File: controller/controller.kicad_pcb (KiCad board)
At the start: 2 copper layers, 160 x 100 mm, 8 parts, among them J2 Barrel_Jack_Switch, J3 Conn_01x02, P1 PMOD-Device-x2-Type-Generic-A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, P2 PMOD-Device-x2-Type-Generic-A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, P3 PMOD-Device-x2-Type-Generic-A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, U1 MAX4820xUP, U3 NUCLEO144-F767ZI, U4 TSR_1-2450

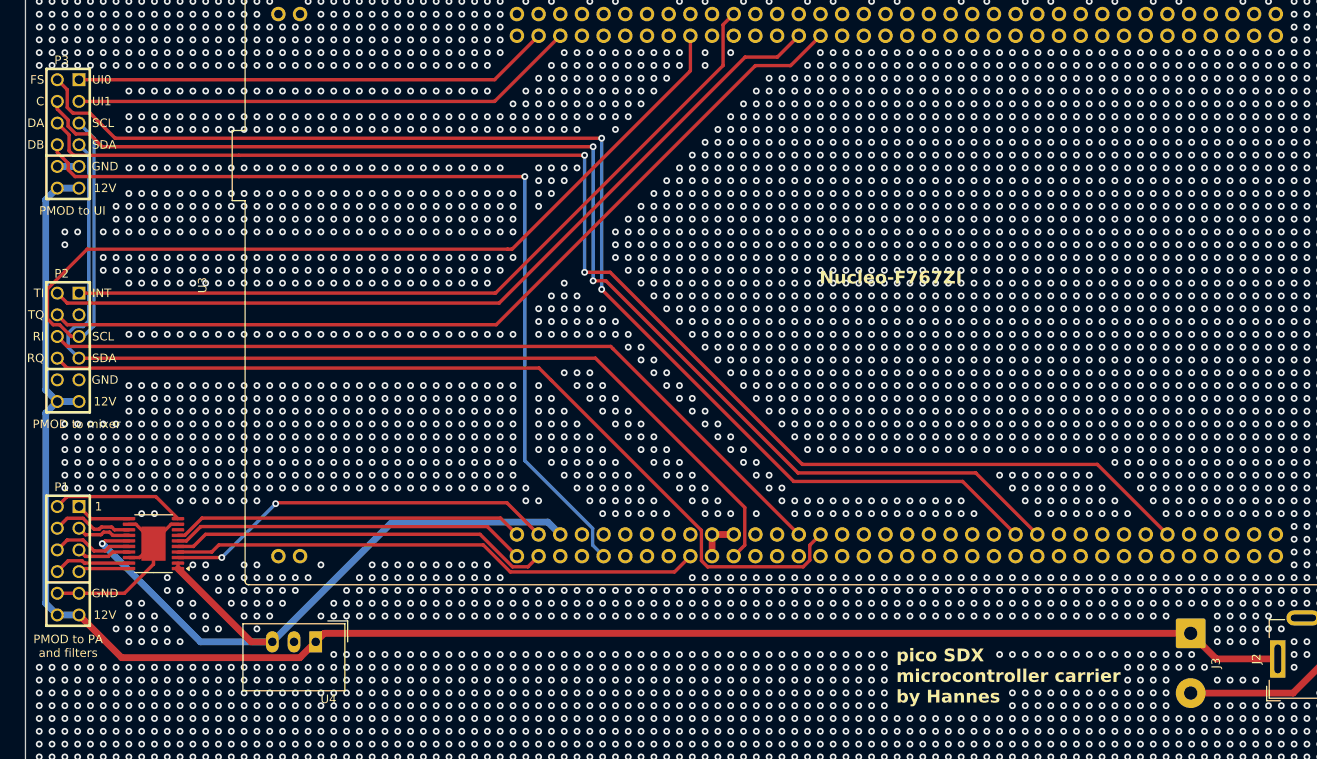
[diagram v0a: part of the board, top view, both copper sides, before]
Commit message: clean up
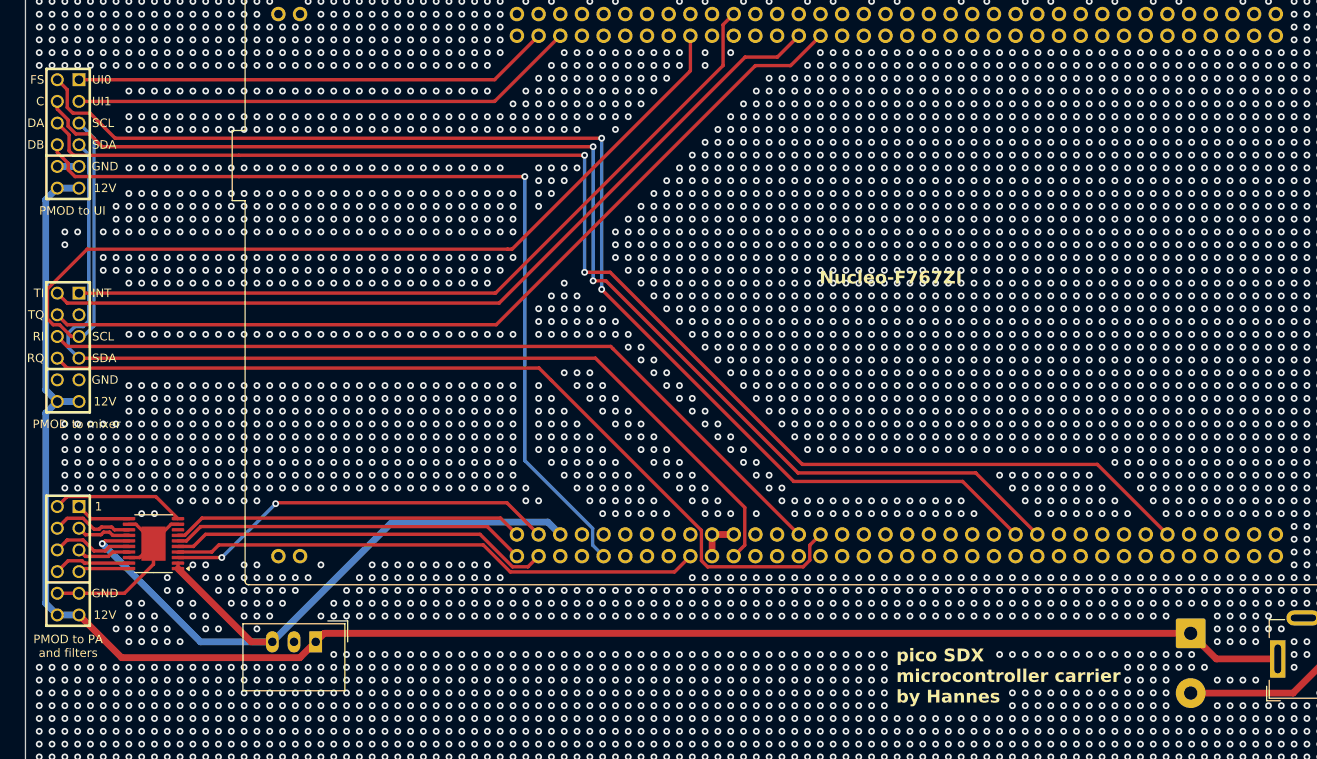
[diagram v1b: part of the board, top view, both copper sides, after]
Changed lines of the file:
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@@
 			(at -1.5 -6.71 0)
 			(layer "F.SilkS")
+			(hide yes)
 			(effects
 				(font
@@
 			(at -0.762 -8.636 0)
 			(layer "F.SilkS")
+			(hide yes)
 			(effects
 				(font
@@
 			(at 3.5 -2.95 90)
 			(layer "F.SilkS")
+			(hide yes)
 			(effects
 				(font
@@
 			(at -0.762 -8.636 0)
 			(layer "F.SilkS")
+			(hide yes)
 			(effects
 				(font
@@
 			(at 0 -2.5 90)
 			(layer "F.SilkS")
+			(hide yes)
 			(effects
 				(font
@@
 			(at -0.762 -8.636 0)
 			(layer "F.SilkS")
+			(hide yes)
 			(effects
 				(font
@@
 			(at 31.75 -36.83 90)
 			(layer "F.SilkS")
+			(hide yes)
 			(effects
 				(font
@@
 		)
 		(height -8)
-		(gr_text "984.2520 mils"
+		(gr_text "25.0000 mm"
 			(at 5.935 42.186 90)
 			(layer "Dwgs.User")
@@
 		)
 		(height -8)
-		(gr_text "984.2520 mils"
+		(gr_text "25.0000 mm"
 			(at 5.935 67.186 90)
 			(layer "Dwgs.User")
@@
 		)
 		(height -8)
-		(gr_text "492.1260 mils"
+		(gr_text "12.5000 mm"
 			(at 5.935 23.436 90)
 			(layer "Dwgs.User")
@@
 		)
 		(height -8)
-		(gr_text "492.1260 mils"
+		(gr_text "12.5000 mm"
 			(at 5.935 98.436 90)
 			(layer "Dwgs.User")
@@
 		)
 		(height -16.5)
-		(gr_text "492.1260 mils"
+		(gr_text "12.5000 mm"
 			(at -2.565 110.936 90)
 			(layer "Dwgs.User")
@@
 		)
 		(height -16.5)
-		(gr_text "984.2520 mils"
+		(gr_text "25.0000 mm"
 			(at -2.565 92.186 90)
 			(layer "Dwgs.User")
